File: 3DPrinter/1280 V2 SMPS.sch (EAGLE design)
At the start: 84 parts, among them IC1 ATMEGA1280-16AU, IC10 TS520533, IC2 7805DT, IC3 CP2102, IC4 X, IC5 Y, IC6 Z, IC7 E0, IC8 E1, IC9 4050D, Q1 16 MHz, X1 USBBF, X2 CON-5.08-03P, X3 CON-5.08-03P, X4 CON-7.62-02P

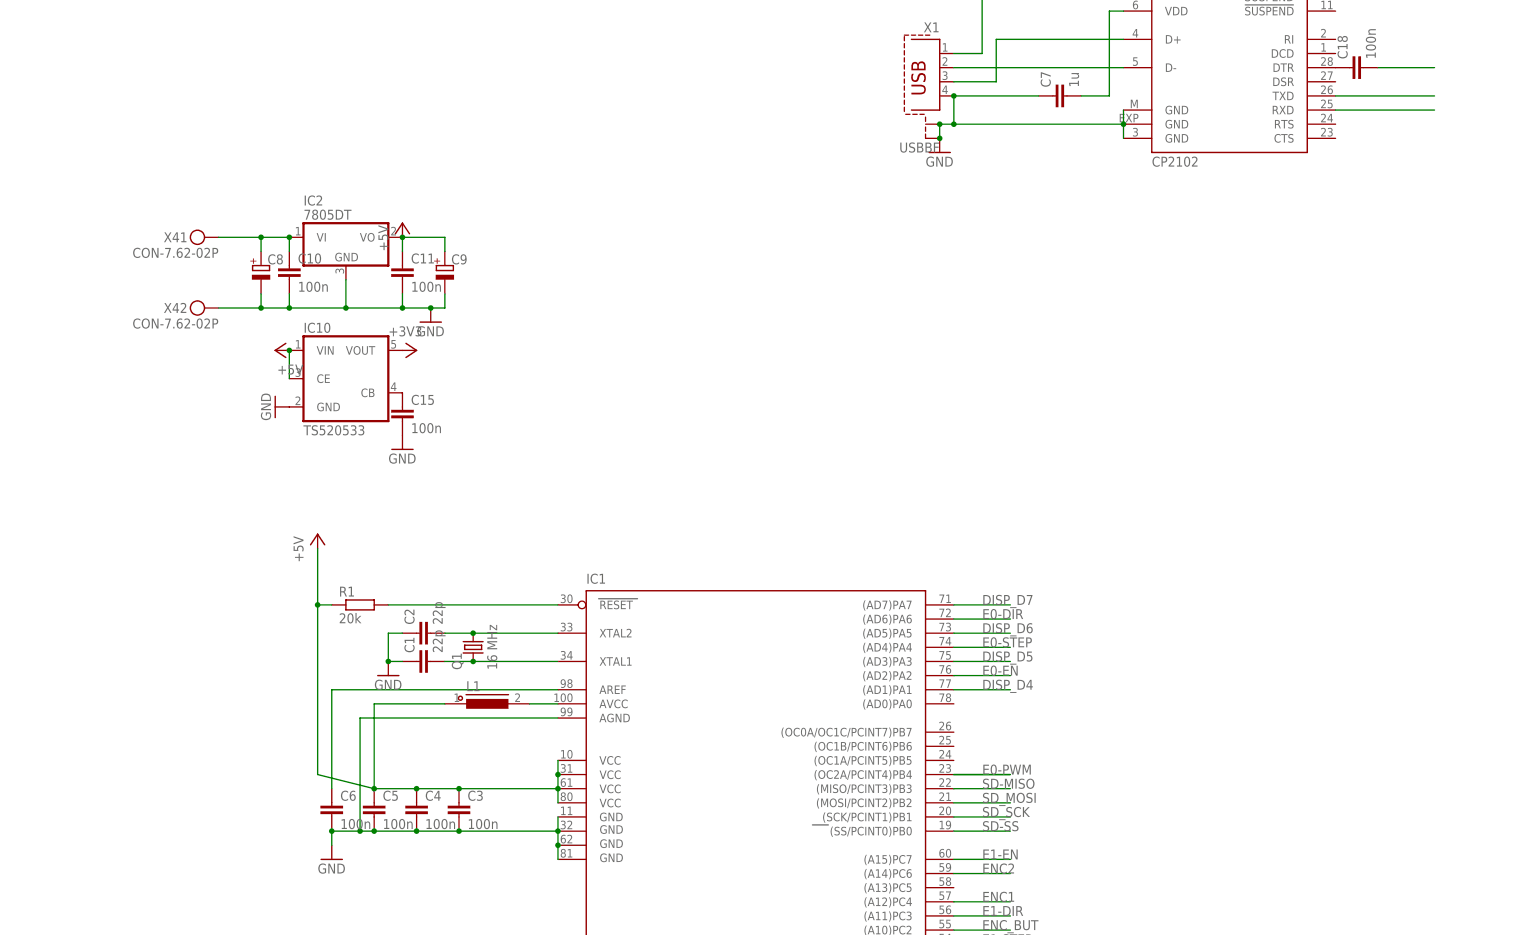
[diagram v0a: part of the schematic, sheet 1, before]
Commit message: SMPS
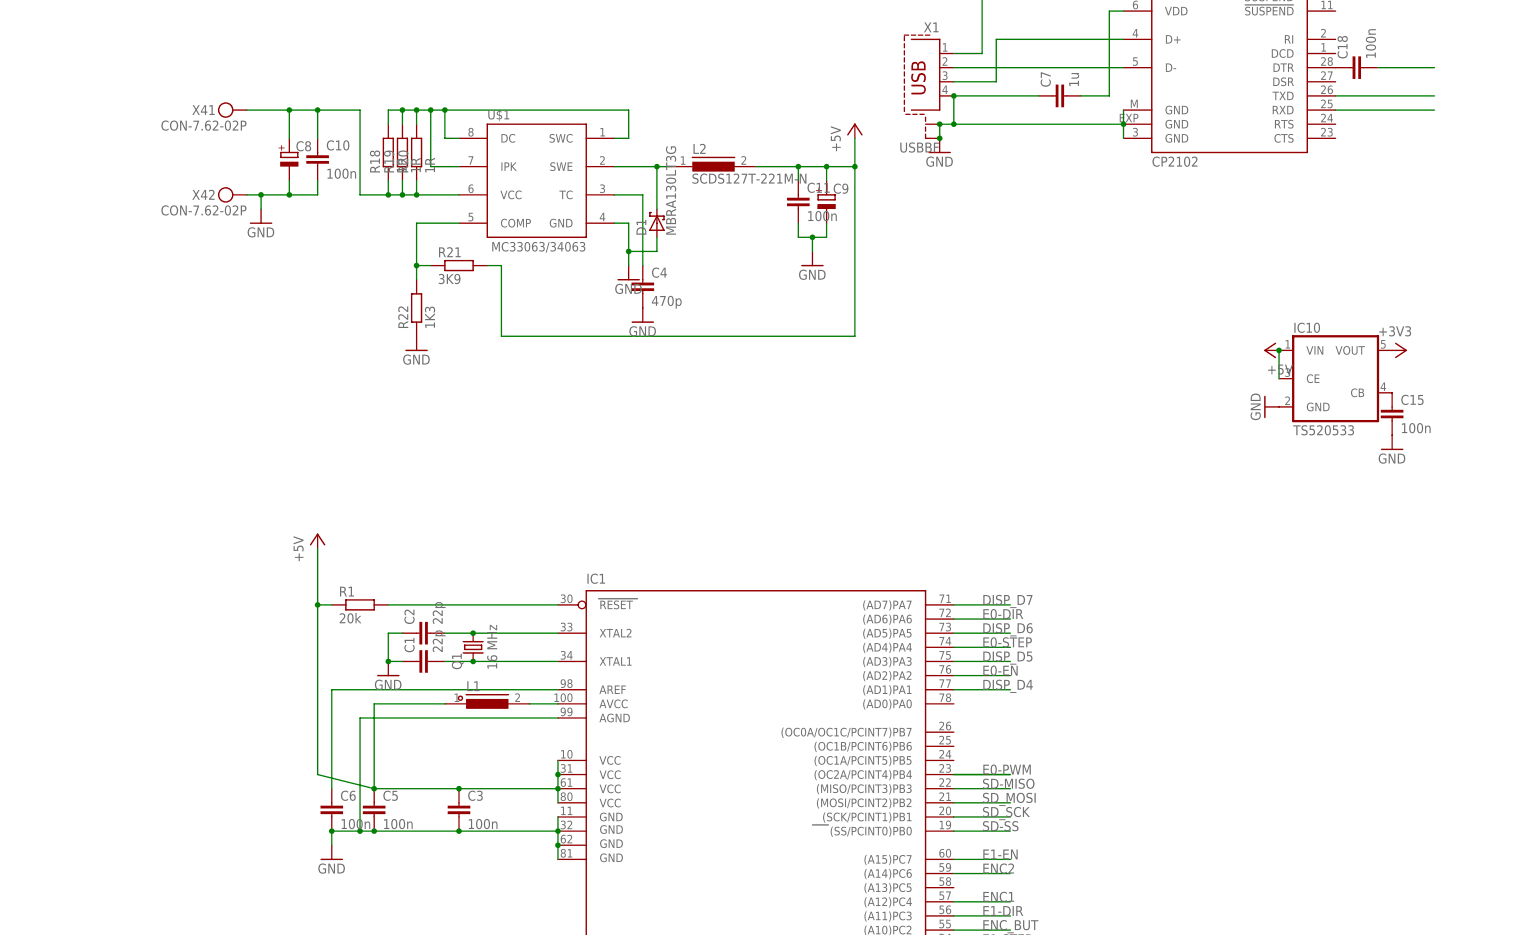
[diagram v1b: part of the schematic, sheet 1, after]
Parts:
- removed IC2: 7805DT, linear:7805DT
- added D1: MBRA130LT3G, Namenlos:DIODE-SH_SMA
- added L2: SCDS127T-221M-N, inductors:DR127
- added R18, R19, R20: 1R, Namenlos:R_0805
- added R21: 3K9, Namenlos:R_0805
- added R22: 1K3, Namenlos:R_0805
- added U$1: MC33063/MC34063D, adafruit:MC33063/MC34063D
- C4: value 100n -> 470p
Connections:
- new net N$47: C10.1, C8.+, R18.1, R19.1, R20.1, U$1.VCC, X41.KL
- new net N$55: R18.2, R19.2, R20.2, U$1.DC, U$1.IPK, U$1.SWC
- new net N$56: D1.C, L2.1, U$1.SWE
- new net N$57: C4.1, U$1.TC
- new net N$59: R21.1, R22.2, U$1.COMP
- net +5V: now also L2.2, R21.2; no longer C4.1, IC2.VO
- net GND: now also D1.A, R22.1, U$1.GND; no longer IC2.GND
- net V-IN: no longer C10.1, C8.+, IC2.VI, X41.KL
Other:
- moved on the sheet: C10, C11, C15, C4, C8, C9, IC10, X41, X42
